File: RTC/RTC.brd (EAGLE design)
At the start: 36.8 x 29.8 mm, 18 parts, among them T1 therm

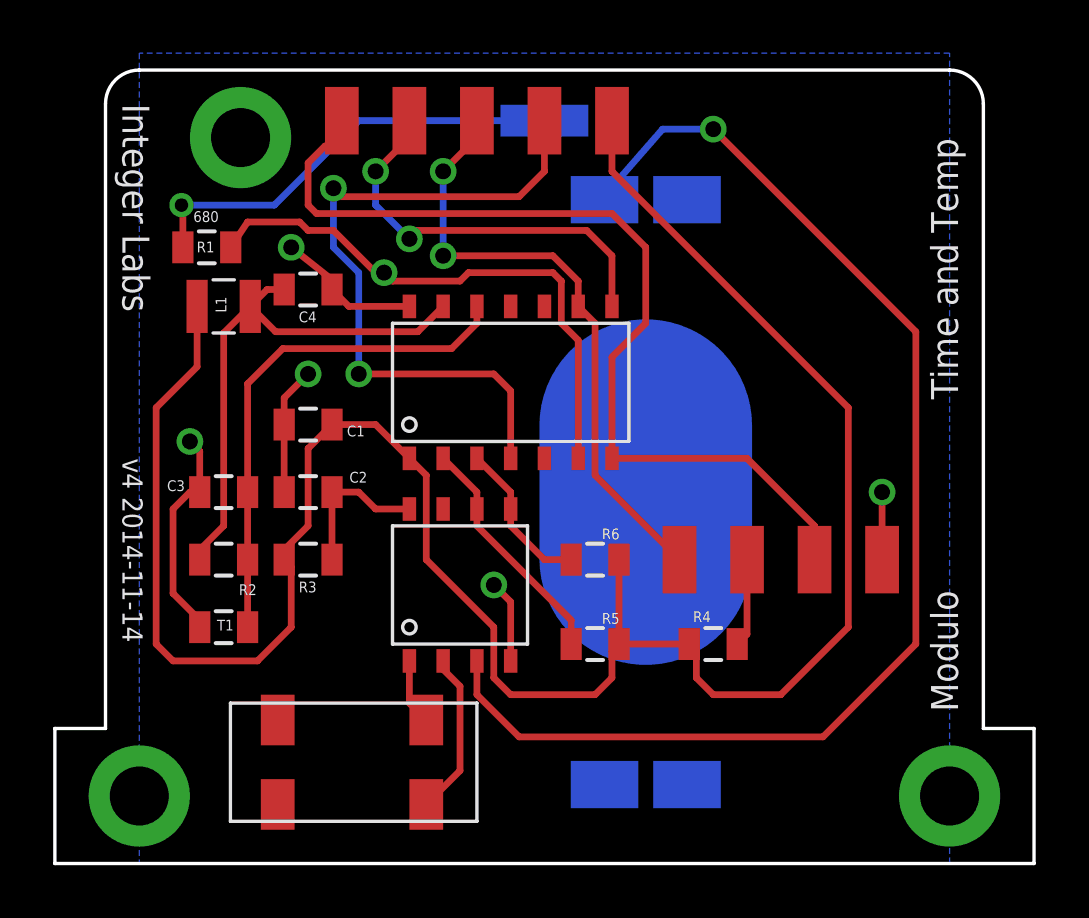
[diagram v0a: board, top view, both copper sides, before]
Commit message: Checkpointing PCB designs
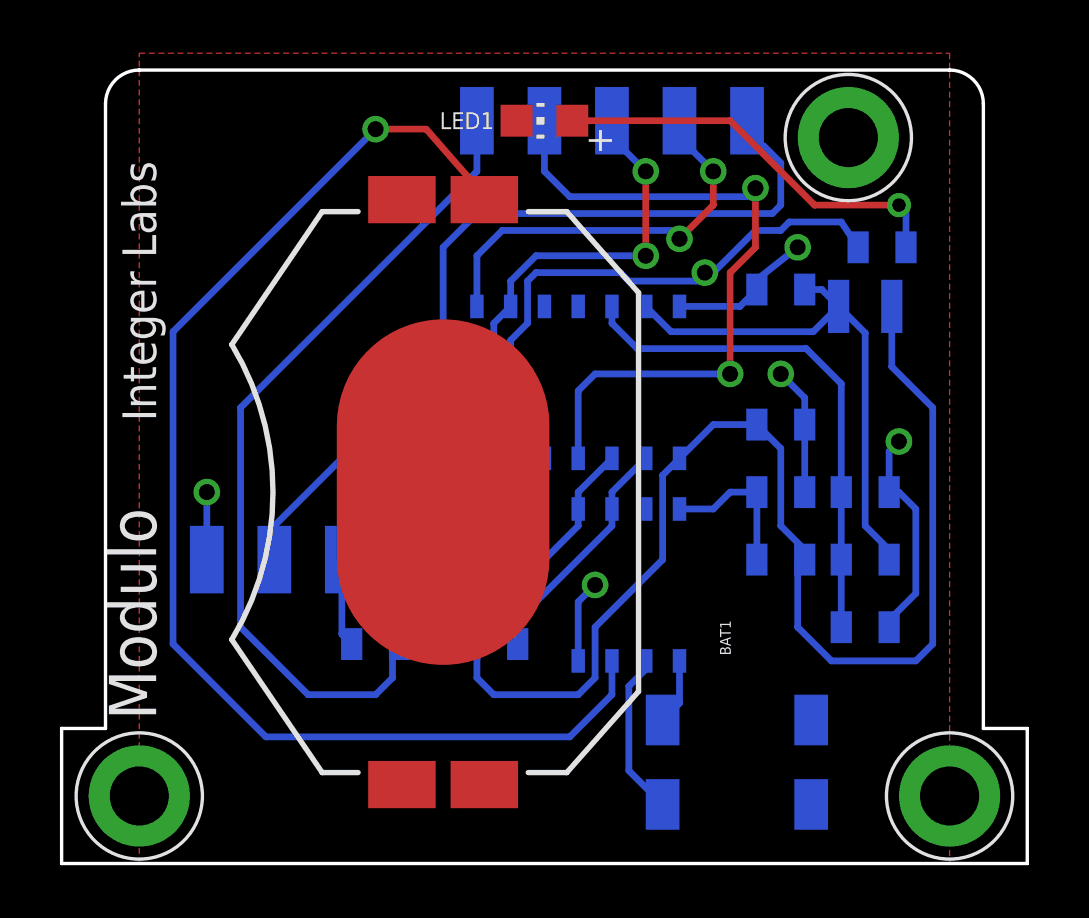
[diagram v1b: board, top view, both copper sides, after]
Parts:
- C2: value 3.3uF -> 10uF
- moved U$4 35.6 mm to (0.00, 0.00), flipped to the top
- moved R1 25.4 mm to (30.5, 23.2), flipped to the bottom
- moved C3 24.1 mm to (29.8, 14.0), flipped to the bottom
- moved L1 24.1 mm to (29.8, 21.0), flipped to the bottom
- moved R2 24.1 mm to (29.8, 11.4), flipped to the bottom
- moved T1 24.1 mm to (29.8, 8.89), flipped to the bottom
- moved C1 17.8 mm to (26.7, 16.5), flipped to the bottom
- moved C2 17.8 mm to (26.7, 14.0), flipped to the bottom
- moved C4 17.8 mm to (26.7, 21.6), flipped to the bottom
- moved R3 17.8 mm to (26.7, 11.4), flipped to the bottom
- moved R4 12.7 mm to (11.4, 8.26), flipped to the bottom
- moved U$3 10.2 mm to (22.9, 18.4), flipped to the bottom
- moved U$1 8.89 mm to (22.2, 5.40), flipped to the bottom
- moved BAT1 7.62 mm to (14.0, 14.0), flipped to the top
- moved U$2 7.62 mm to (21.6, 10.8), flipped to the bottom
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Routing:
- added copper zone on layer 1, net GND
- removed copper zone on layer 16, net GND
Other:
- board size 36.8 x 29.8 mm -> 36.3 x 29.8 mm
- board text removed: "Integer Labs"
- board text removed: "Modulo"
- board text removed: "Time and Temp"
- board text removed: "v4 2014-11-14"
